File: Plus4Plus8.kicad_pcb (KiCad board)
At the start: 2 copper layers, 22 parts, among them CN1 JOY1, CN2 JOY2, CN3 JOY3, CN4 JOY4, CN5 JOY5, CN6 JOY6, CN7 JOY7, CN8 JOY8, CN9 PLUS4_USERPORT, U1 CD4051B, U2 CD4051B, U3 CD4051B, U4 CD4051B, U5 CD4051B

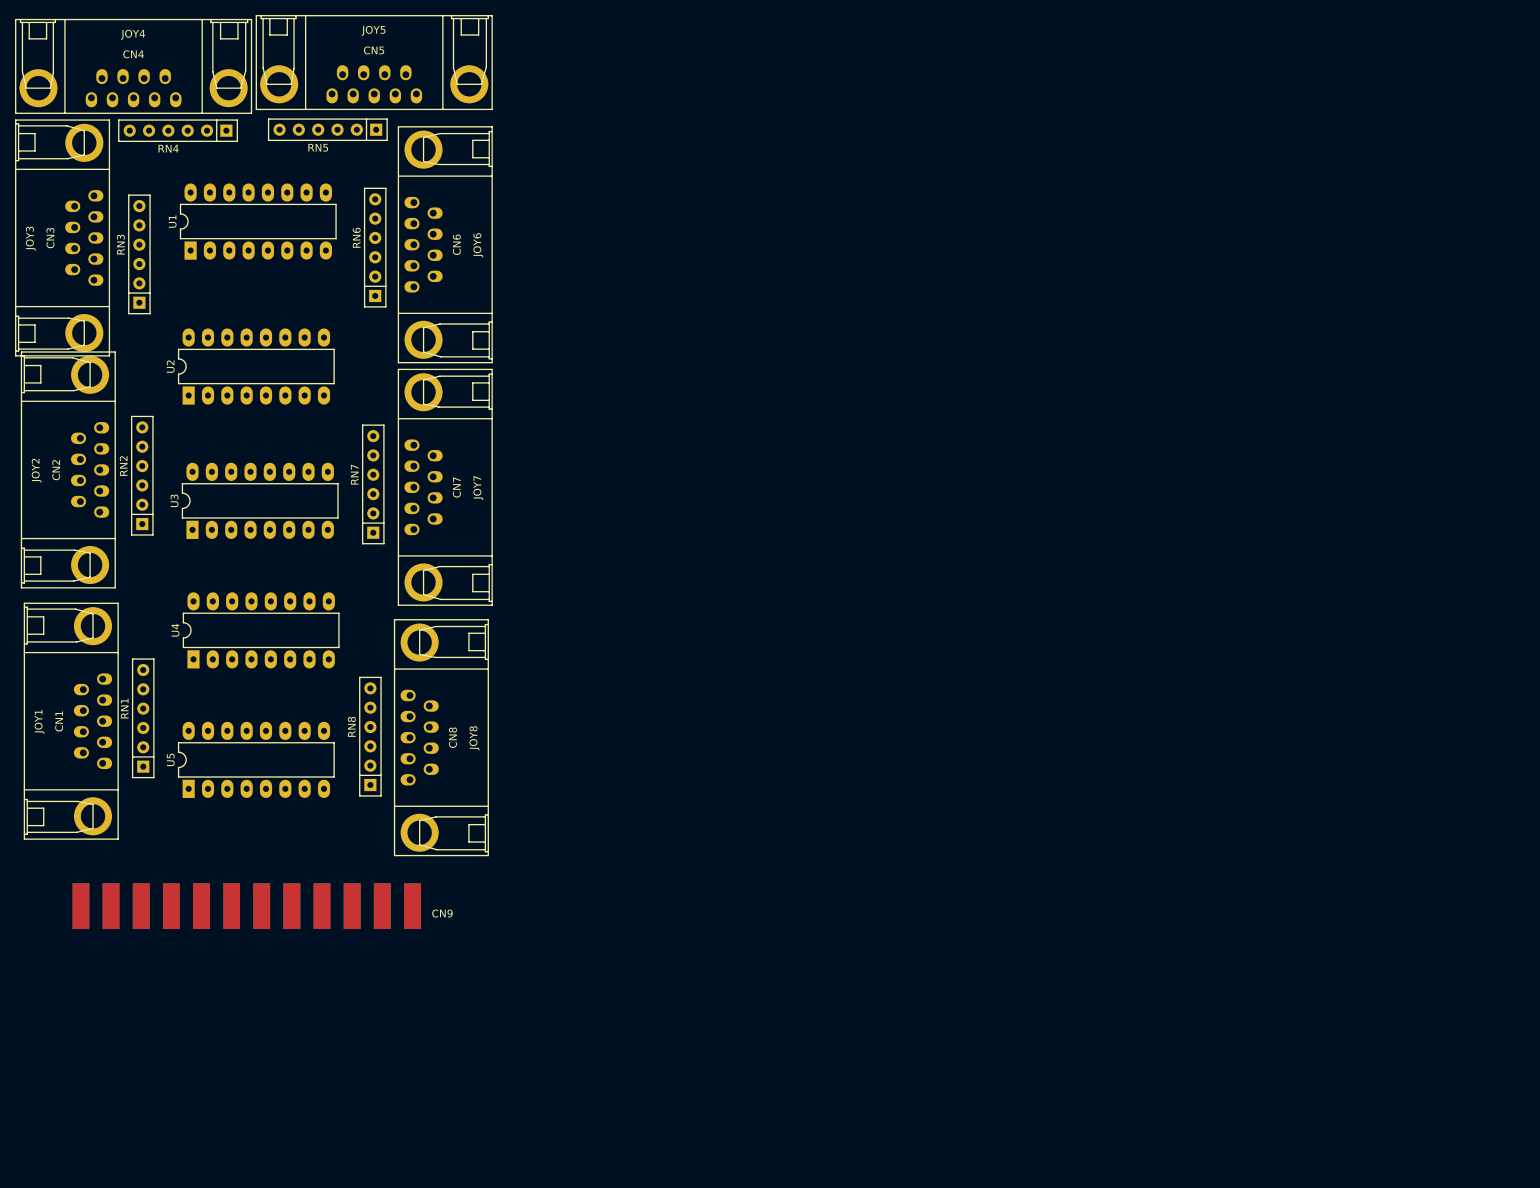
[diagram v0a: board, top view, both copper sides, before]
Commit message: Initial layout
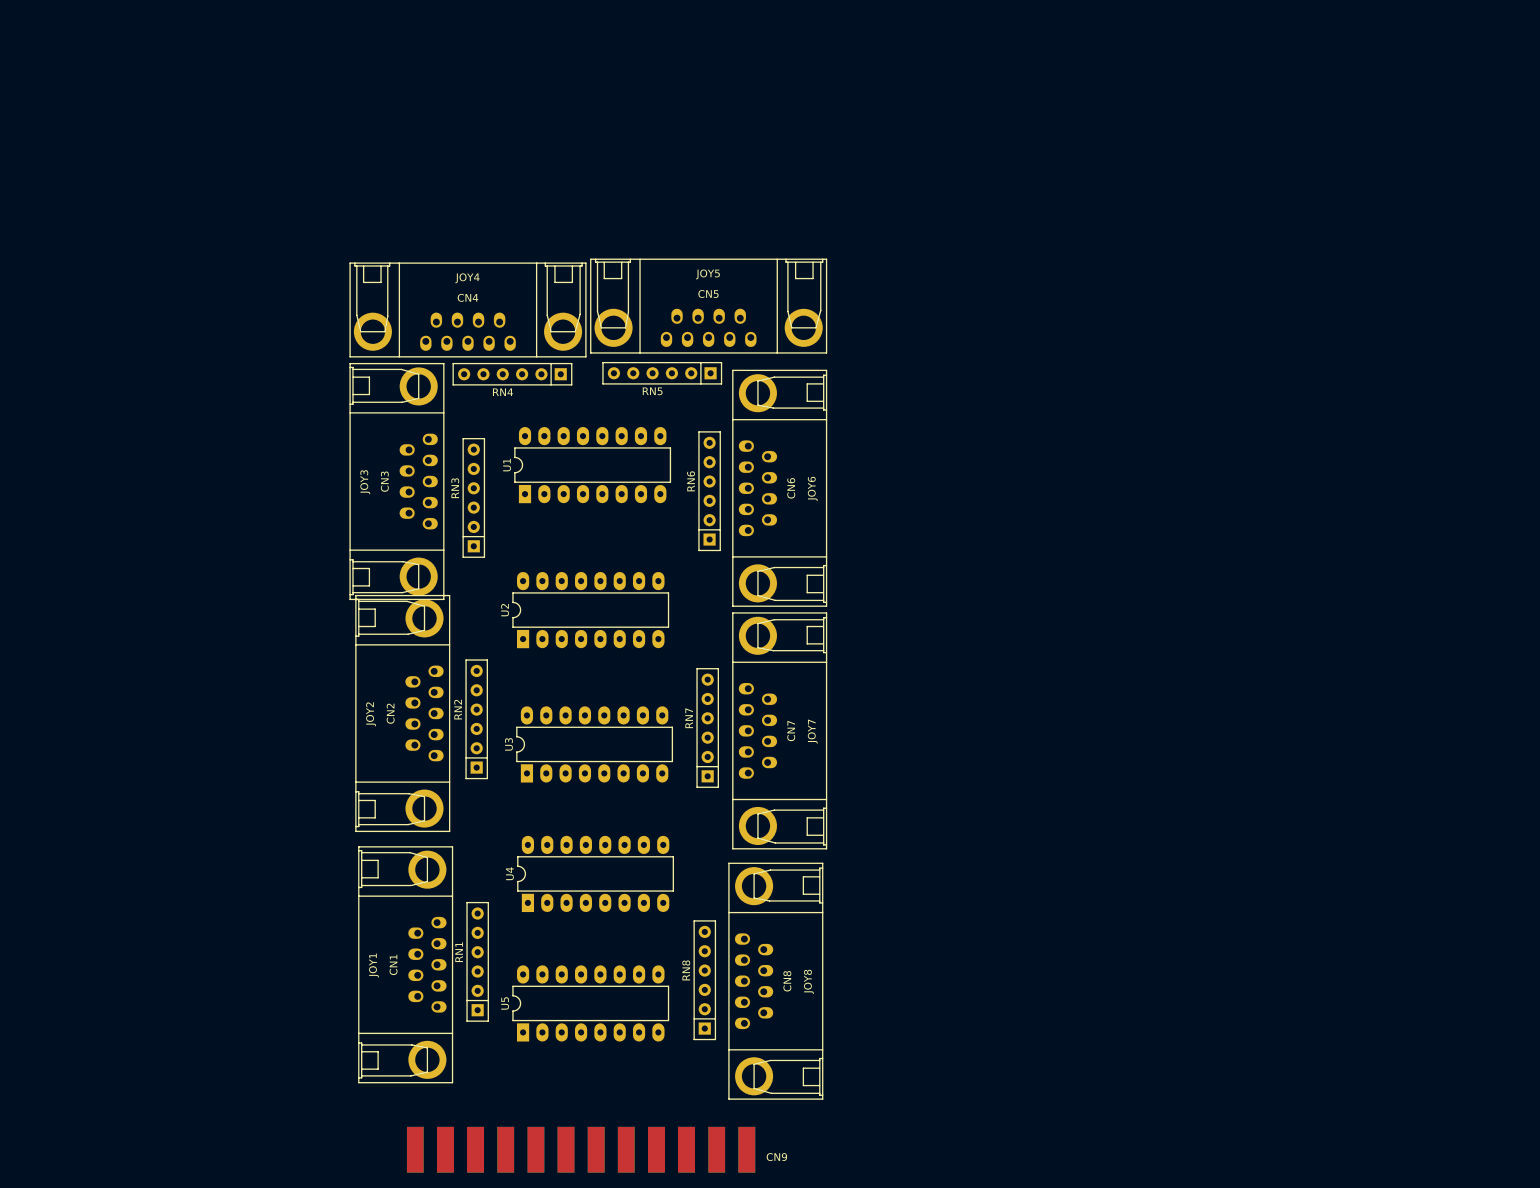
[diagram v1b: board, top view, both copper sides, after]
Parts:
- moved CN1 54.4 mm to (130.9, 121.8)
- moved CN2 54.4 mm to (130.6, 88.8)
- moved CN3 54.4 mm to (129.8, 58.3)
- moved CN4 54.4 mm to (143.4, 31.5)
- moved CN5 54.4 mm to (175.0, 31.0)
- moved CN6 54.4 mm to (188.6, 59.2)
- moved CN7 54.4 mm to (188.6, 91.1)
- moved CN9 54.4 mm to (158.2, 149.1)
- moved RN2 54.4 mm to (144.5, 95.9)
- moved RN3 54.4 mm to (144.1, 66.8)
- moved RN6 54.4 mm to (175.1, 65.9)
- moved U1 54.4 mm to (150.9, 59.9)
- moved U2 54.4 mm to (150.6, 79.0)
- moved U4 54.4 mm to (151.3, 113.7)
- moved U5 54.4 mm to (150.6, 130.7)
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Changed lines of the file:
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@@
   )
   (module Plus4Plus8:DB_9M (layer F.Cu)
-    (at 86.995 89.789 270)
+    (at 130.937 121.793 270)
     (descr "D-SUB 9 pin plug, Tyco P/N 4-338168-2")
     (fp_text reference CN1 (at 0 -2.7 90) (layer F.SilkS)
@@
   )
   (module Plus4Plus8:DB_9M (layer F.Cu)
-    (at 86.614 56.769 270)
+    (at 130.556 88.773 270)
     (descr "D-SUB 9 pin plug, Tyco P/N 4-338168-2")
     (fp_text reference CN2 (at 0 -2.7 90) (layer F.SilkS)
@@
   )
   (module Plus4Plus8:DB_9M (layer F.Cu)
-    (at 85.852 26.289 270)
+    (at 129.794 58.293 270)
     (descr "D-SUB 9 pin plug, Tyco P/N 4-338168-2")
     (fp_text reference CN3 (at 0 -2.7 90) (layer F.SilkS)
@@
   )
   (module Plus4Plus8:DB_9M (layer F.Cu)
-    (at 99.441 -0.508 180)
+    (at 143.383 31.496 180)
     (descr "D-SUB 9 pin plug, Tyco P/N 4-338168-2")
     (fp_text reference CN4 (at 0 -2.7) (layer F.SilkS)
@@
   )
   (module Plus4Plus8:DB_9M (layer F.Cu)
-    (at 131.064 -1.016 180)
+    (at 175.006 30.988 180)
     (descr "D-SUB 9 pin plug, Tyco P/N 4-338168-2")
     (fp_text reference CN5 (at 0 -2.7) (layer F.SilkS)
@@
   )
   (module Plus4Plus8:DB_9M (layer F.Cu)
-    (at 144.653 27.178 90)
+    (at 188.595 59.182 90)
     (descr "D-SUB 9 pin plug, Tyco P/N 4-338168-2")
     (fp_text reference CN6 (at 0 -2.7 90) (layer F.SilkS)
@@
   )
   (module Plus4Plus8:DB_9M (layer F.Cu)
-    (at 144.653 59.055 90)
+    (at 188.595 91.059 90)
     (descr "D-SUB 9 pin plug, Tyco P/N 4-338168-2")
     (fp_text reference CN7 (at 0 -2.7 90) (layer F.SilkS)
@@
   )
   (module Plus4Plus8:DB_9M (layer F.Cu)
-    (at 144.145 91.948 90)
+    (at 188.087 123.952 90)
     (descr "D-SUB 9 pin plug, Tyco P/N 4-338168-2")
     (fp_text reference CN8 (at 0 -2.7 90) (layer F.SilkS)
@@
   )
   (module Plus4Plus8:PLUS4_USERPORT (layer F.Cu)
-    (at 114.3 117.094)
+    (at 158.242 149.098)
     (attr smd)
     (fp_text reference CN9 (at 25.74 -2) (layer F.SilkS)
@@
   )
   (module Resistor_THT:R_Array_SIP6 (layer F.Cu)
-    (at 100.711 95.758 90)
+    (at 144.653 127.762 90)
     (descr "6-pin Resistor SIP pack")
     (tags R)
@@
   )
   (module Resistor_THT:R_Array_SIP6 (layer F.Cu)
-    (at 100.584 63.881 90)
+    (at 144.526 95.885 90)
     (descr "6-pin Resistor SIP pack")
     (tags R)
@@
   )
   (module Resistor_THT:R_Array_SIP6 (layer F.Cu)
-    (at 100.203 34.798 90)
+    (at 144.145 66.802 90)
     (descr "6-pin Resistor SIP pack")
     (tags R)
@@
   )
   (module Resistor_THT:R_Array_SIP6 (layer F.Cu)
-    (at 111.633 12.192 180)
+    (at 155.575 44.196 180)
     (descr "6-pin Resistor SIP pack")
     (tags R)
@@
   )
   (module Resistor_THT:R_Array_SIP6 (layer F.Cu)
-    (at 131.318 12.065 180)
+    (at 175.26 44.069 180)
     (descr "6-pin Resistor SIP pack")
     (tags R)
@@
   )
   (module Resistor_THT:R_Array_SIP6 (layer F.Cu)
-    (at 131.191 33.909 90)
+    (at 175.133 65.913 90)
     (descr "6-pin Resistor SIP pack")
     (tags R)
@@
   )
   (module Resistor_THT:R_Array_SIP6 (layer F.Cu)
-    (at 130.937 65.024 90)
+    (at 174.879 97.028 90)
     (descr "6-pin Resistor SIP pack")
     (tags R)
@@
   )
   (module Resistor_THT:R_Array_SIP6 (layer F.Cu)
-    (at 130.556 98.171 90)
+    (at 174.498 130.175 90)
     (descr "6-pin Resistor SIP pack")
     (tags R)
@@
   )
   (module Package_DIP:DIP-16_W7.62mm_LongPads (layer F.Cu)
-    (at 106.934 27.94 90)
+    (at 150.876 59.944 90)
     (descr "16-lead though-hole mounted DIP package, row spacing 7.62 mm (300 mils), LongPads")
     (tags "THT DIP DIL PDIP 2.54mm 7.62mm 300mil LongPads")
@@
   )
   (module Package_DIP:DIP-16_W7.62mm_LongPads (layer F.Cu)
-    (at 106.68 46.99 90)
+    (at 150.622 78.994 90)
     (descr "16-lead though-hole mounted DIP package, row spacing 7.62 mm (300 mils), LongPads")
     (tags "THT DIP DIL PDIP 2.54mm 7.62mm 300mil LongPads")
@@
   )
   (module Package_DIP:DIP-16_W7.62mm_LongPads (layer F.Cu)
-    (at 107.188 64.643 90)
+    (at 151.13 96.647 90)
     (descr "16-lead though-hole mounted DIP package, row spacing 7.62 mm (300 mils), LongPads")
     (tags "THT DIP DIL PDIP 2.54mm 7.62mm 300mil LongPads")
@@
   )
   (module Package_DIP:DIP-16_W7.62mm_LongPads (layer F.Cu)
-    (at 107.315 81.661 90)
+    (at 151.257 113.665 90)
     (descr "16-lead though-hole mounted DIP package, row spacing 7.62 mm (300 mils), LongPads")
     (tags "THT DIP DIL PDIP 2.54mm 7.62mm 300mil LongPads")
@@
   )
   (module Package_DIP:DIP-16_W7.62mm_LongPads (layer F.Cu)
-    (at 106.68 98.679 90)
+    (at 150.622 130.683 90)
     (descr "16-lead though-hole mounted DIP package, row spacing 7.62 mm (300 mils), LongPads")
     (tags "THT DIP DIL PDIP 2.54mm 7.62mm 300mil LongPads")

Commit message: New layout, way funnier
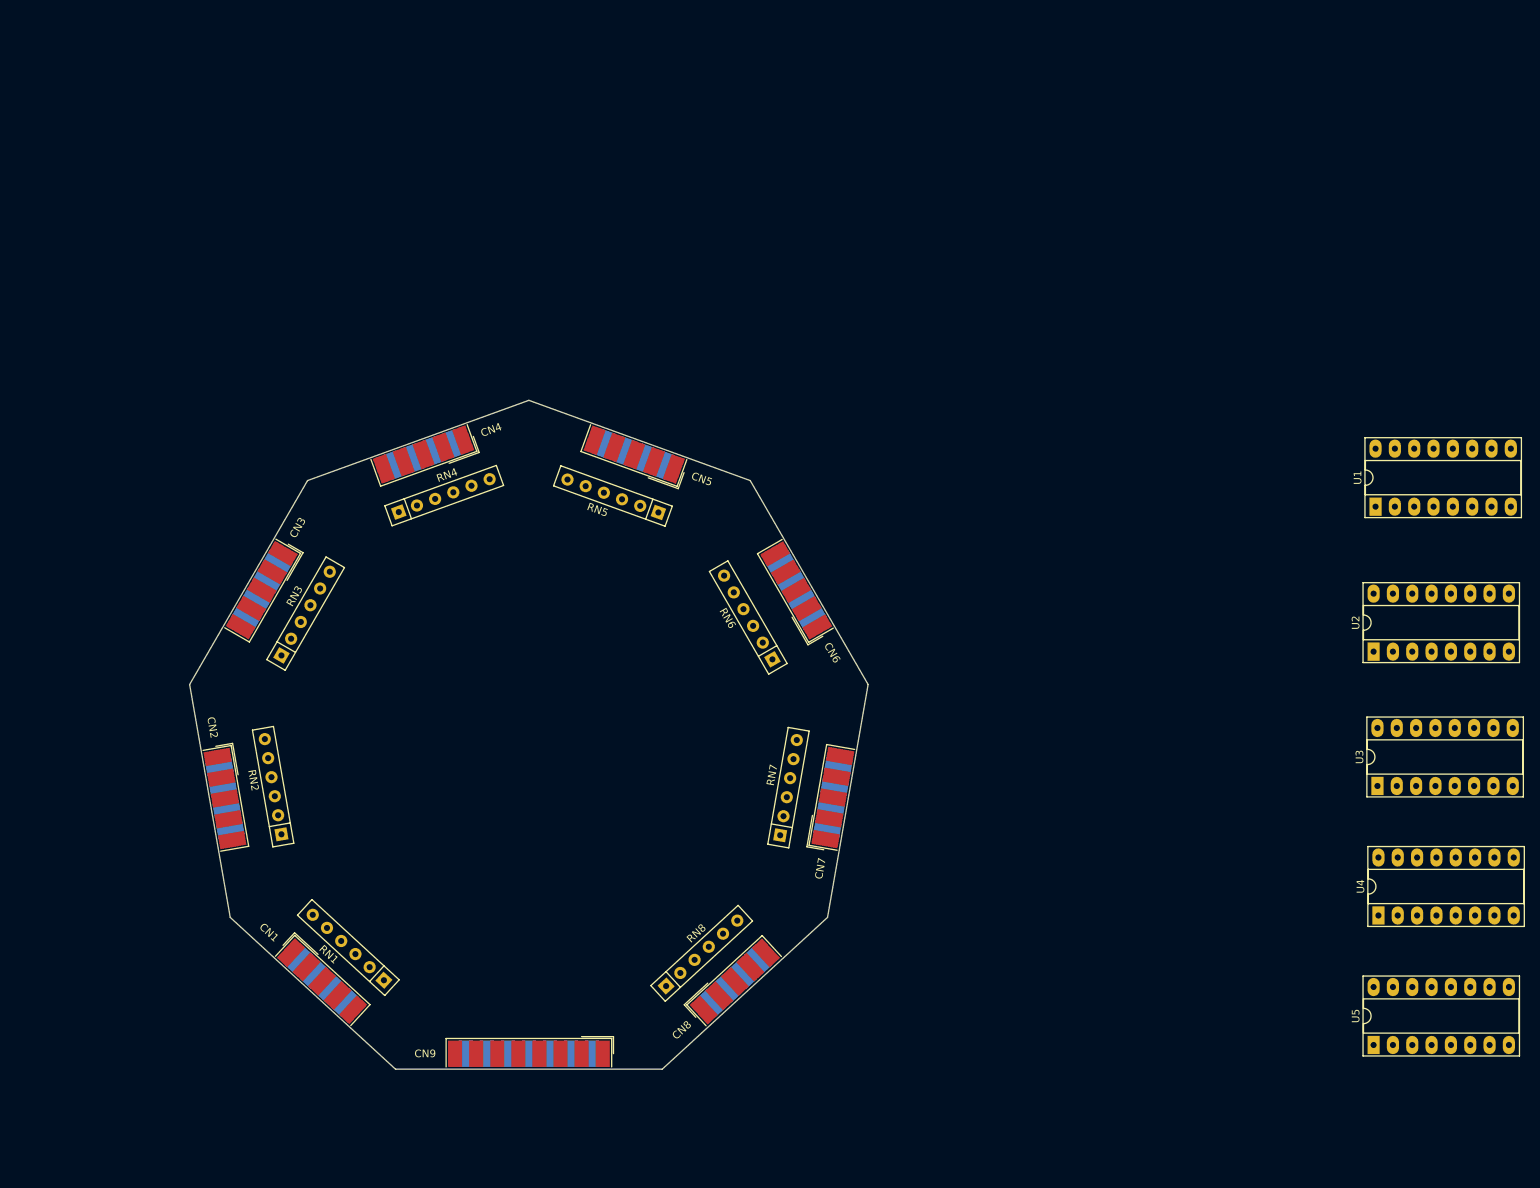
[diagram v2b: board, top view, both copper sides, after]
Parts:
- CN1, CN2, CN3, CN4, CN5, CN6, CN7, CN8: footprint Plus4Plus8:DB_9M -> Connector_Dsub:DSUB-9_Male_EdgeMount_P2.77mm
- CN9: value PLUS4_USERPORT -> DB15F; footprint Plus4Plus8:PLUS4_USERPORT -> Connector_Dsub:DSUB-15_Female_EdgeMount_P2.77mm
- U1, U2, U3, U4, U5: footprint Package_DIP:DIP-16_W7.62mm_LongPads -> Package_DIP:DIP-16_W7.62mm_Socket_LongPads
- moved U1 111.8 mm to (262.6, 61.6)
- moved U2 111.8 mm to (262.4, 80.6)
- moved U3 111.8 mm to (262.9, 98.3)
- moved U4 111.8 mm to (263.0, 115.3)
- moved U5 111.8 mm to (262.4, 132.3)
- moved RN3 29.1 mm to (118.9, 81.1), turned to 60 degrees
- moved RN4 27.9 mm to (134.3, 62.3), turned to 19.9 degrees
- moved RN2 27.1 mm to (118.9, 104.6), turned to 99.9 degrees
- moved CN5 25.7 mm to (165.2, 54.8), turned to 160.1 degrees
- moved CN4 24.0 mm to (137.5, 54.7), turned to 199.9 degrees
- moved CN2 22.1 mm to (111.4, 99.9), turned to 279.9 degrees
- moved CN3 19.6 mm to (116.3, 72.6), turned to 240 degrees
- moved RN5 19.5 mm to (168.4, 62.4), turned to 160.1 degrees
- moved RN6 17.8 mm to (183.4, 81.7), turned to 120 degrees
- moved CN9 17.1 mm to (151.4, 133.5)
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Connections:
- CN9 pad 1: GND -> +5V
- CN9 pad 10: (no net) -> /d4
- CN9 pad 11: (no net) -> /d5
- CN9 pad 12: GND -> /d6
- CN9 pad 2: +5V -> /d0
- CN9 pad 3: (no net) -> /d1
- CN9 pad 6: /d4 -> (no net)
- CN9 pad 7: /d5 -> (no net)
- CN9 pad 8: (no net) -> GND
- CN9 pad 9: (no net) -> +5V
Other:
- board outline added: 89.2 x 87.9 mm
